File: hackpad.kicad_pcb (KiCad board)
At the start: 2 copper layers, 104.8 x 61.9 mm, 32 parts, among them J1 OLED Connection, SW1 SW_Push, SW11 RotaryEncoder_Switch, SW13 RotaryEncoder_Switch, SW2 SW_Push, SW3 SW_Push, SW4 SW_Push, SW5 SW_Push, SW6 SW_Push, SW7 SW_Push, SW8 SW_Push, U1 XIAO-RP2040-DIP

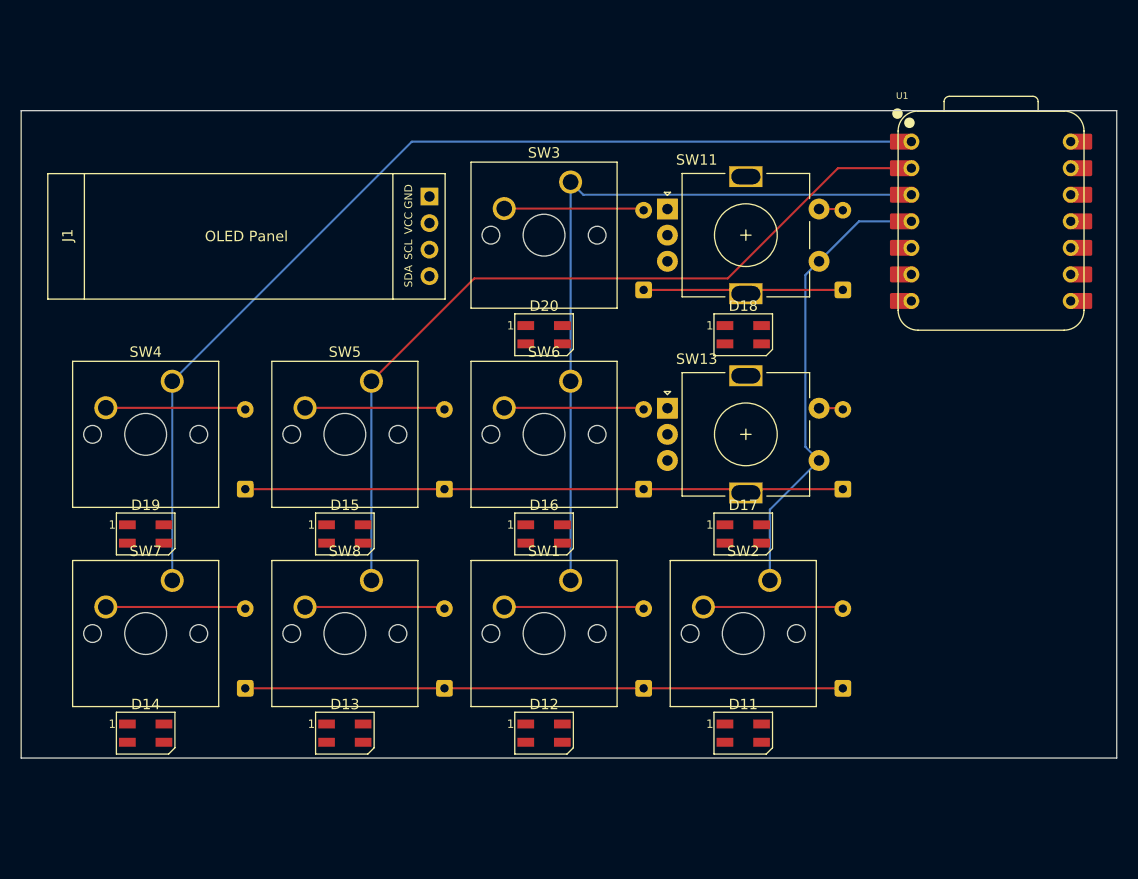
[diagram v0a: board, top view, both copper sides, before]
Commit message: finish pcb
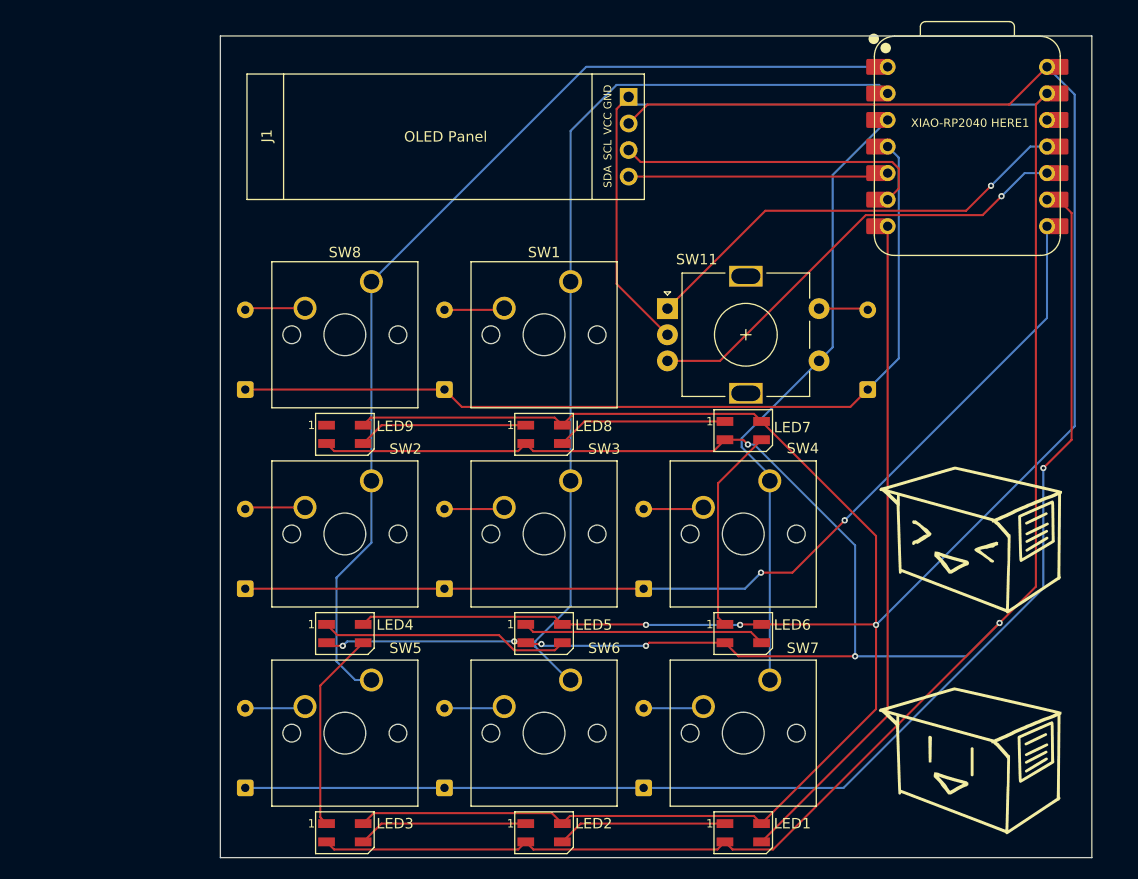
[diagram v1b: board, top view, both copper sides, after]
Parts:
- removed D10, D9: 1N4148, Diode_THT:D_DO-35_SOD27_P7.62mm_Horizontal
- removed D12, D13, D14, D15, D16, D17, D18, D19, D20: SK6812MINI, LED_SMD:LED_SK6812MINI_PLCC4_3.5x3.5mm_P1.75mm
- removed SW13: RotaryEncoder_Switch, Rotary_Encoder:RotaryEncoder_Alps_EC11E-Switch_Vertical_H20mm
- removed U1: XIAO-RP2040-DIP, OPL:XIAO-RP2040-DIP
- added G***: LOGO, Images:tv2, F.Cu at (137.0, 116.0)
- added G***: LOGO, Images:tv, F.Cu at (136.9, 137.1)
- added LED1: SK6812MINI, LED_SMD:LED_SK6812MINI_PLCC4_3.5x3.5mm_P1.75mm, F.Cu at (114.3, 142.9)
- added LED2: SK6812MINI, LED_SMD:LED_SK6812MINI_PLCC4_3.5x3.5mm_P1.75mm, F.Cu at (95.2, 142.9)
- added LED3: SK6812MINI, LED_SMD:LED_SK6812MINI_PLCC4_3.5x3.5mm_P1.75mm, F.Cu at (76.2, 142.9)
- added LED4: SK6812MINI, LED_SMD:LED_SK6812MINI_PLCC4_3.5x3.5mm_P1.75mm, F.Cu at (76.2, 123.8)
- added LED5: SK6812MINI, LED_SMD:LED_SK6812MINI_PLCC4_3.5x3.5mm_P1.75mm, F.Cu at (95.2, 123.8)
- added LED6: SK6812MINI, LED_SMD:LED_SK6812MINI_PLCC4_3.5x3.5mm_P1.75mm, F.Cu at (114.3, 123.8)
- added LED7: SK6812MINI, LED_SMD:LED_SK6812MINI_PLCC4_3.5x3.5mm_P1.75mm, F.Cu at (114.3, 104.4)
- added LED8: SK6812MINI, LED_SMD:LED_SK6812MINI_PLCC4_3.5x3.5mm_P1.75mm, F.Cu at (95.2, 104.8)
- added LED9: SK6812MINI, LED_SMD:LED_SK6812MINI_PLCC4_3.5x3.5mm_P1.75mm, F.Cu at (76.2, 104.8)
- added XIAO-RP2040 HERE1: XIAO-RP2040-DIP, OPL:XIAO-RP2040-DIP, F.Cu at (135.7, 77.2)
- added anime: LOGO, Images:anime, B.Cu at (127.0, 124.0)
- D11: value SK6812MINI -> 1N4148; footprint LED_SMD:LED_SK6812MINI_PLCC4_3.5x3.5mm_P1.75mm -> Diode_THT:D_DO-35_SOD27_P7.62mm_Horizontal; moved to B.Cu
- moved D2 57.9 mm to (66.7, 119.5)
- moved SW4 57.9 mm to (116.8, 109.2)
- moved SW7 57.9 mm to (116.8, 128.3)
- moved D7 39.3 mm to (104.8, 138.6)
- moved SW2 39.3 mm to (78.7, 109.2)
- moved D4 39.3 mm to (104.8, 119.5)
- moved D11 35.0 mm to (126.2, 100.5), turned to 90 degrees
- moved D1 34.3 mm to (85.7, 100.5)
- moved D6 34.3 mm to (85.7, 138.6)
- moved D3 34.3 mm to (85.7, 119.5)
- moved D5 34.3 mm to (66.7, 138.6)
- moved D8 34.3 mm to (66.7, 100.5)
- moved SW5 28.6 mm to (78.7, 128.3)
- moved SW6 28.6 mm to (97.8, 128.3)
- moved SW1 28.6 mm to (97.8, 90.2)
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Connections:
- D1 pad 1: Row 2 -> Row 0
- D11 pad 1: Net-(D11-DOUT) -> Row 0
- D11 pad 2: GND -> SW11S2
- D2 pad 1: Row 2 -> Row 1
- D3 pad 1: Row 0 -> Row 1
- D5 pad 1: Row 1 -> Row 2
- D6 pad 1: Row 1 -> Row 2
- D8 pad 1: Row 2 -> Row 0
- J1 pad 2: VCC -> +5V
- SW1 pad 1: Column 2 -> Column 1
- SW11 pad S1: Column 3 -> Column 2
- SW2 pad 1: Column 3 -> Column 0
- SW3 pad 1: Column 2 -> Column 1
- SW4 pad 1: Column 0 -> Column 2
- SW5 pad 1: Column 1 -> Column 0
- SW6 pad 1: Column 2 -> Column 1
- SW7 pad 1: Column 0 -> Column 2
- SW8 pad 1: Column 1 -> Column 0
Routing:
- net GND: track 0.00 -> 326.9 mm, vias 0 -> 7
- net +5V: track 0.00 -> 280.8 mm, vias 0 -> 3
- net Row 2: track 57.2 -> 124.1 mm, vias 0 -> 1
- net Row 0: track 19.0 -> 85.8 mm
- net LED: track 0.00 -> 63.9 mm
- net Column 3: track 44.0 -> 0.00 mm
- net SW11B: track 0.00 -> 43.7 mm, vias 0 -> 1
- net SW11A: track 0.00 -> 42.7 mm, vias 0 -> 1
- net Row 1: track 57.2 -> 96.2 mm, vias 0 -> 2
- net SCL: track 0.00 -> 30.0 mm
- net SDA: track 0.00 -> 24.9 mm
- net Net-(LED4-DOUT): track 0.00 -> 23.9 mm
- net Net-(LED5-DOUT): track 0.00 -> 23.3 mm
- net Net-(LED6-DOUT): track 0.00 -> 19.7 mm
- net Net-(LED3-DOUT): track 0.00 -> 19.2 mm
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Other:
- board size 104.8 x 61.9 mm -> 83.3 x 78.6 mm
